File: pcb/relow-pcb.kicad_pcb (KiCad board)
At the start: 2 copper layers, 76.2 x 44.5 mm, 71 parts, among them IC1 AD8495, IC2 ATMEGA328P_TQFP, IC3 FT230X_SOP, J1 MICROUSB, J2 TOASTER, K1 S212S01, P1 AVR_ISP, Q1 MMBT4401, Q2 MMBT4401, Q3 MMBT4401, Q4 MMBT4401, Q5 MMBT4401

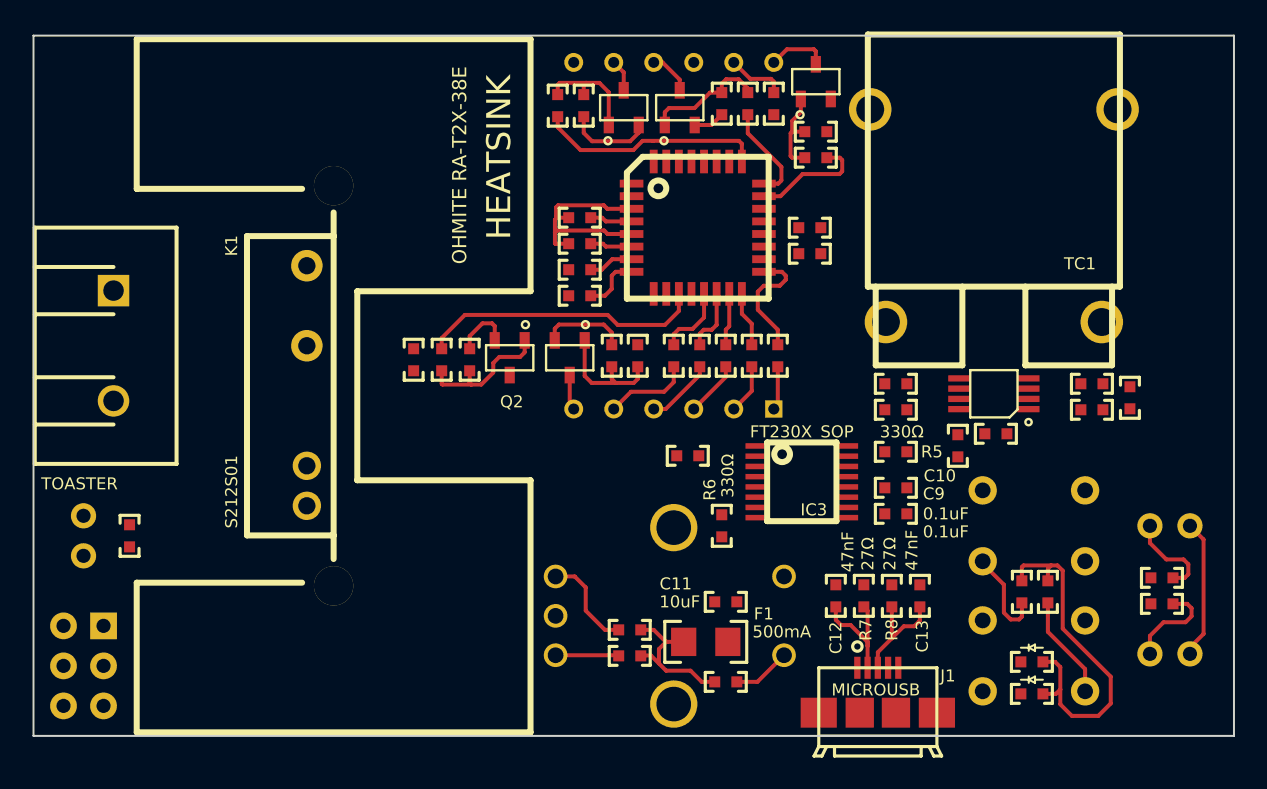
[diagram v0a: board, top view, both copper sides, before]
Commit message: layout done. ready to order (after triple checking)
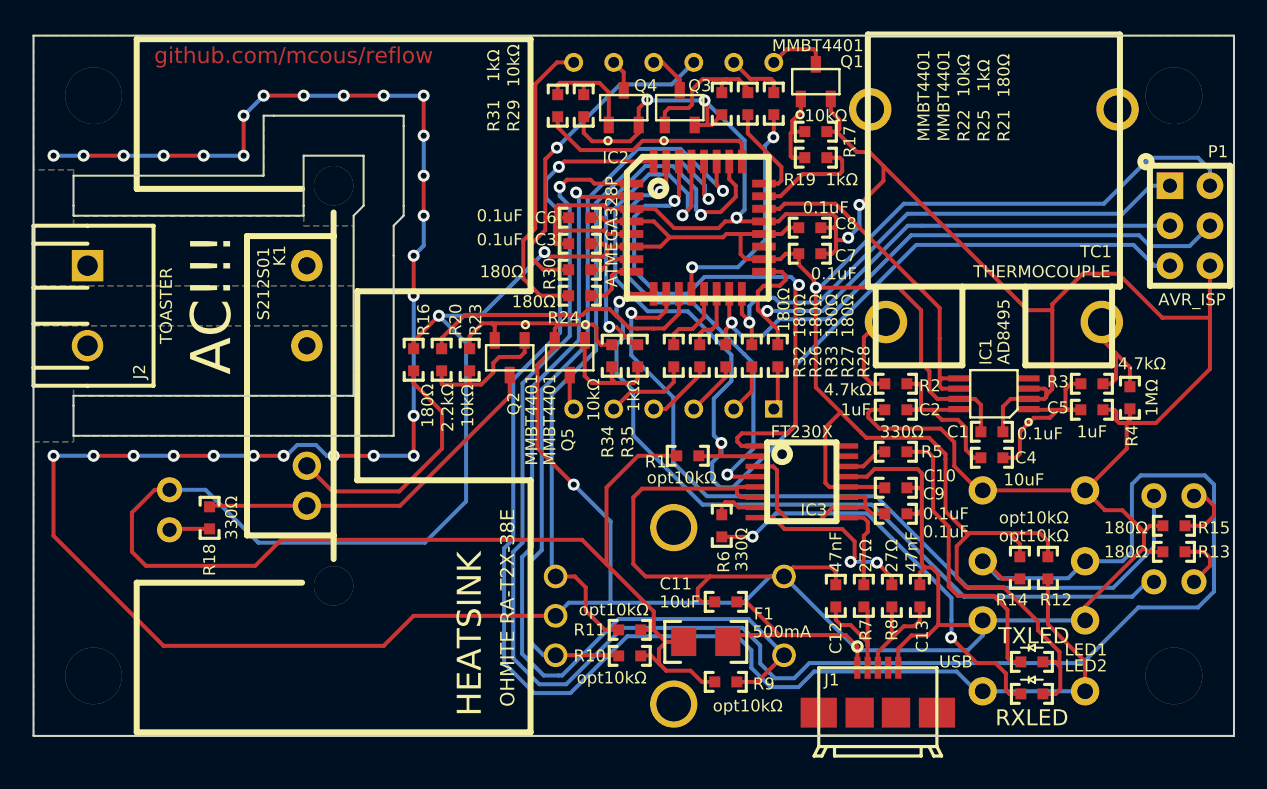
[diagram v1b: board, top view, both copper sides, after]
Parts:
- added M3: VAL**, M3, B.Cu at (172.1, 160.0)
- added M3: VAL**, M3, B.Cu at (172.1, 123.2)
- added M3: VAL**, M3, B.Cu at (103.5, 160.0)
- added M3: VAL**, M3, B.Cu at (103.5, 123.2)
- IC2: value ATMEGA328P_TQFP -> ATMEGA328P
- IC3: value FT230X_SOP -> FT230X
- J1: value MICROUSB -> USB
- J2: footprint 2-PIN_SCREW-TERM_P7.5MM -> 2-PIN_SCREW-TERM_P200MIL
- P1: moved to F.Cu
- R1, R10, R11, R12, R14, R9: value 10kΩ_opt -> opt10kΩ
- moved P1 75.6 mm to (173.1, 131.4), turned to 0 degrees
- moved LED5 5.71 mm to (108.3, 149.5)
- moved R18 5.21 mm to (110.9, 150.0)
- moved LED3 4.58 mm to (172.1, 154.1)
- moved R13 3.39 mm to (172.1, 152.1), turned to 0 degrees
- moved R15 3.39 mm to (172.1, 150.5), turned to 0 degrees
- moved J2 3.03 mm to (103.1, 136.5)
- moved C1 2.33 mm to (160.5, 144.5), turned to 180 degrees
- moved LED4 1.92 mm to (172.1, 148.6)
- moved C4 1.55 mm to (160.5, 146.2)
- moved R14 1.53 mm to (162.3, 153.2)
- moved R12 1.52 mm to (164.1, 153.2)
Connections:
- LED3 pad 1: GND -> N-000002
- LED3 pad 2: N-000002 -> /LED_START
- LED4 pad 1: GND -> N-000003
- LED4 pad 2: N-000003 -> /LED_STOP
- R13 pad 1: N-000002 -> GND
- R13 pad 2: /LED_START -> N-000002
- R15 pad 1: N-000003 -> GND
- R15 pad 2: /LED_STOP -> N-000003
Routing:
- net GND: track 39.4 -> 403.1 mm, vias 0 -> 34
- net VCC: track 38.5 -> 242.9 mm, vias 0 -> 3
- net /STOP: track 6.09 -> 117.7 mm, vias 0 -> 1
- net /START: track 6.59 -> 90.0 mm, vias 0 -> 1
- net /RESET: track 0.00 -> 76.7 mm, vias 0 -> 2
- net /SET: track 3.70 -> 57.9 mm, vias 0 -> 1
- net /LED_STOP: track 0.00 -> 52.3 mm, vias 0 -> 1
- net /LED_START: track 0.00 -> 49.4 mm, vias 0 -> 1
- net /ENC_A: track 4.02 -> 48.6 mm, vias 0 -> 1
- net /ENC_B: track 6.27 -> 43.5 mm, vias 0 -> 1
- net /USART_RX: track 0.00 -> 35.3 mm, vias 0 -> 2
- net /MOSI: track 3.32 -> 37.9 mm, vias 0 -> 1
- net /MISO: track 3.49 -> 34.8 mm, vias 0 -> 1
- net /USART_TX: track 0.00 -> 28.9 mm, vias 0 -> 2
- net /SCK: track 7.73 -> 36.1 mm, vias 0 -> 1
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- added copper zone on B.Cu, net GND
- added copper zone on F.Cu, net GND
- added copper zone on B.Cu, net N-0000049
- added copper zone on F.Cu, net N-0000049
- added copper zone on B.Cu, net N-0000051
- added copper zone on F.Cu, net N-0000051
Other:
- outline, holes or cut-outs redrawn
- board text added: "<-AC!!!"
- board text added: "AC!!!"
- board text added: "CUT OUT"
- board text added: "github.com/mcous/reflow"
- board text added: "github.com/mcous/reflow open source hardware cc by-sa 3.0 mjc 11/5/13"
- board text added: "push to select"
